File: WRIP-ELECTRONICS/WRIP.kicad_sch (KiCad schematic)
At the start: 22 parts, among them J1 Conn_01x02_Pin, J3 Conn_01x02_Pin, J4 Conn_01x01_Pin, J5 Conn_01x01_Pin, J6 Conn_01x01_Pin, J7 Conn_01x01_Pin, J8 Conn_01x01_Pin, SW1 SW_Push

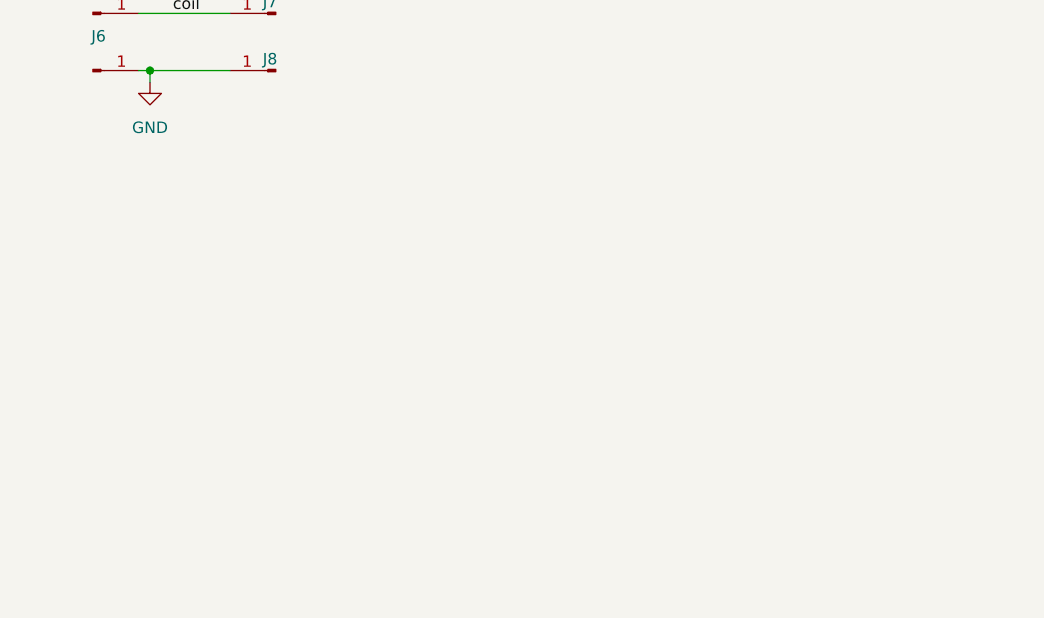
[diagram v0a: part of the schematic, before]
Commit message: JBH
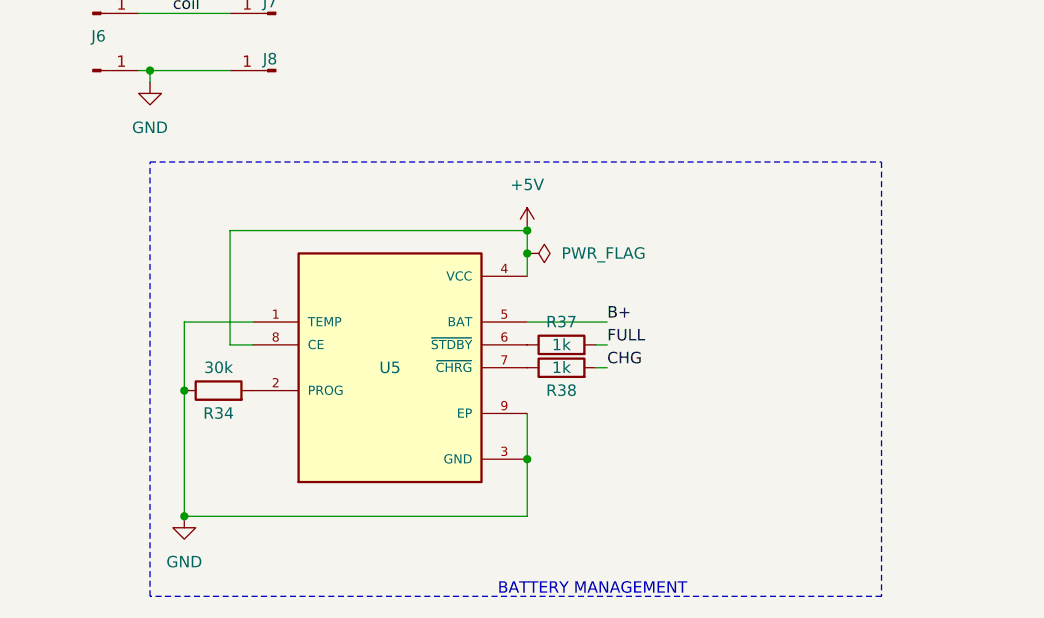
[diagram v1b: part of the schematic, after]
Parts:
- added R34: 30k, Resistor_SMD:R_0603_1608Metric, symbol Device:R
- added R37, R38: 1k, Resistor_SMD:R_0603_1608Metric, symbol Device:R
- added U5: TP4056, Package_SO:SOIC-8-1EP_3.9x4.9mm_P1.27mm_EP2.41x3.3mm_ThermalVias, symbol 1_sfxer symbols:IC_Battery_Management{colon}SOP-8_TP4056
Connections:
- net GND: now also R34.1, U5.1 (TEMP), U5.3 (GND), U5.9 (EP)
- new net: R34.2, U5.2 (PROG)
- new net: R37.1, U5.6 (~{STDBY})
- new net: R38.1, U5.7 (~{CHRG})
- new net +5V: U5.4 (VCC), U5.8 (CE)
- new net B+: U5.5 (BAT)
- new net CHG: R38.2
- new net FULL: R37.2
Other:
- note added: "BATTERY MANAGEMENT"
